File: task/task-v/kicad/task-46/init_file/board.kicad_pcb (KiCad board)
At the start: 2 copper layers, 80 x 80 mm, 8 parts

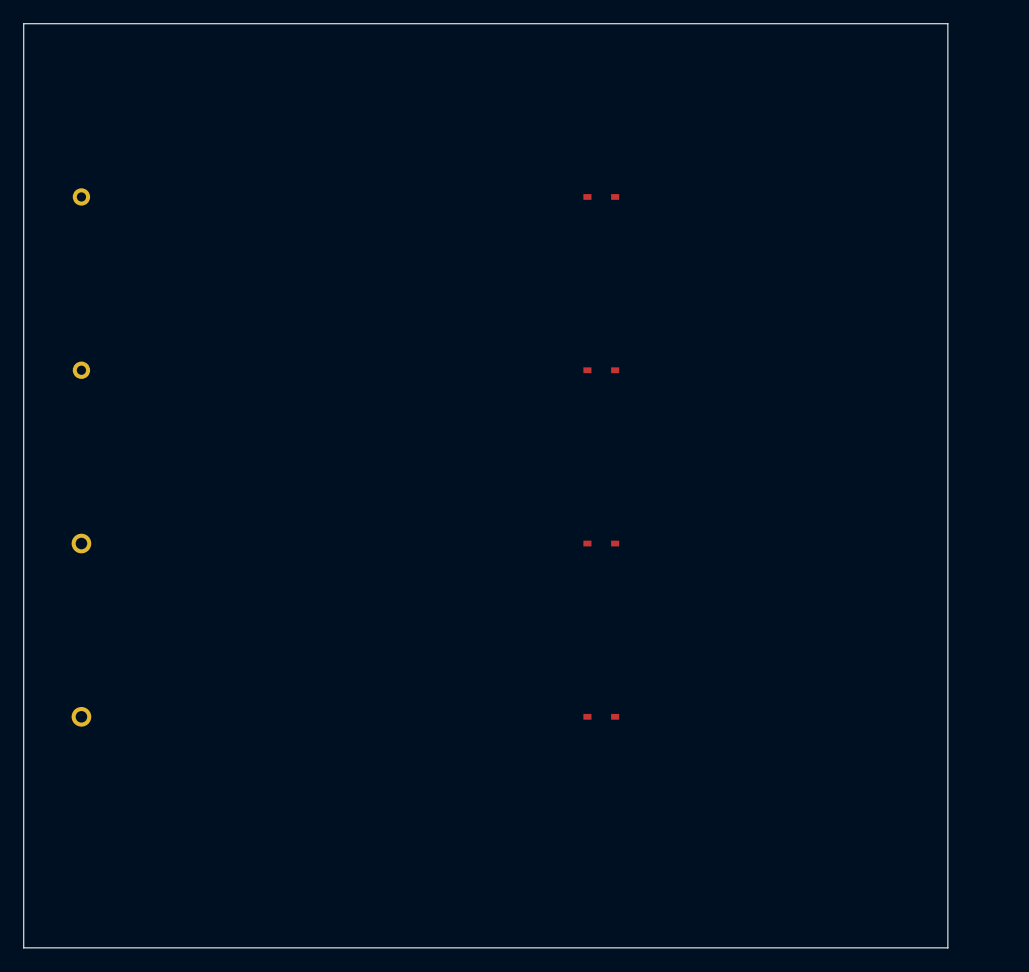
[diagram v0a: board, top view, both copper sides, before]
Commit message: Refine engineering task metadata and instructions
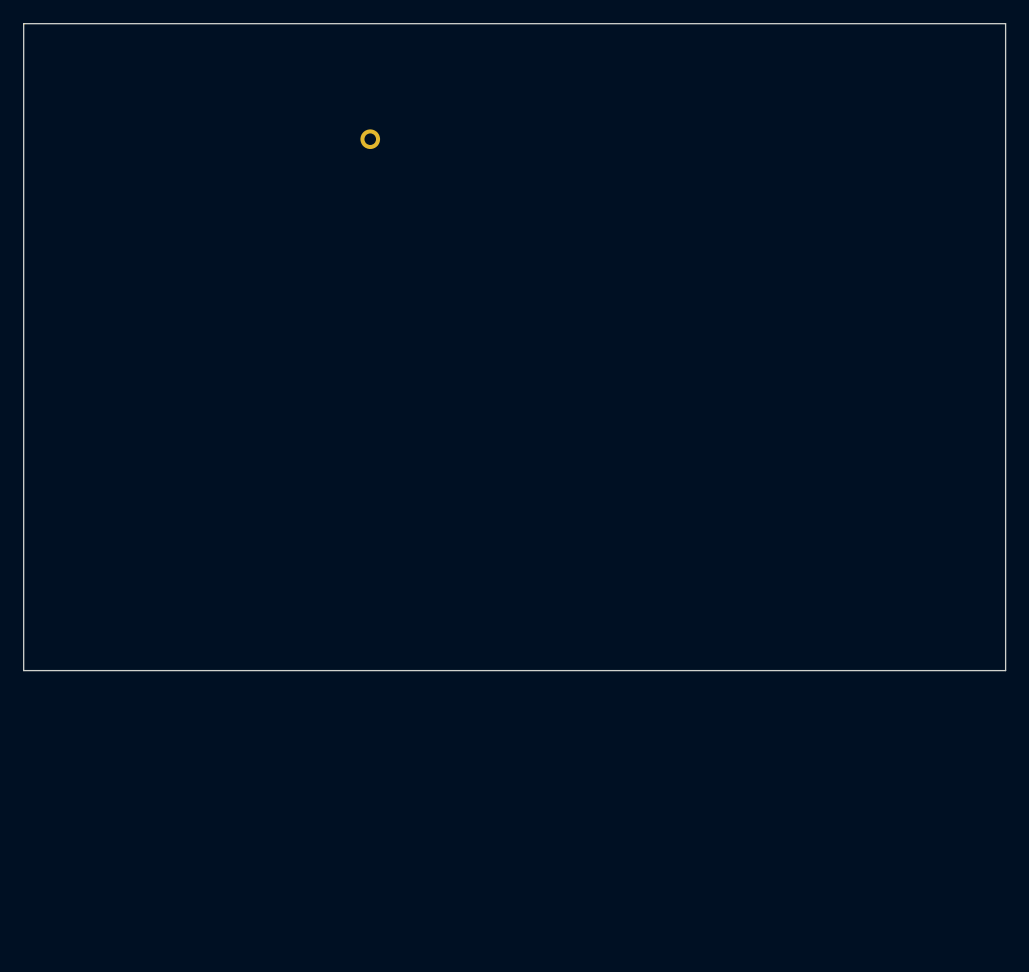
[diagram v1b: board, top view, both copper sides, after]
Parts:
- removed the ? at (5.00, 15.0)
- removed the ? at (5.00, 30.0)
- removed the ? at (5.00, 45.0)
- removed the ? at (5.00, 60.0)
- removed the ? at (50.0, 15.0)
- removed the ? at (50.0, 30.0)
- removed the ? at (50.0, 45.0)
- removed the ? at (50.0, 60.0)
- added ?: , Connector_PinHeader_2.54mm:PinHeader_2x20_P2.54mm_Vertical, F.Cu at (30.0, 10.0)
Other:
- board size 80 x 80 mm -> 85 x 56 mm
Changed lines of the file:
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@@
   )
   (net 0 "")
-  (net 1 "USB_DP")
-  (net 2 "USB_DM")
-  (net 3 "SIG_TX")
-  (net 4 "SIG_RX")
-  (net 5 "GND")
-  ; Connectors at board edge (x=5)
-  (footprint "Connector_USB:USB_A_Molex_67643_Vertical" (layer "F.Cu") (at 5 15)
-    (reference "J1") (value "USB-A")
-    (pad "1" thru_hole circle (at 0 0) (size 1.5 1.5) (drill 0.8)
-      (layers "F.Cu" "B.Cu" "F.Mask" "B.Mask") (net 1 "USB_DP"))
+  (net 1 "VCC")
+  (net 2 "GND")
+  ; Initial board: 85x56mm rectangle, no mounting holes, no rounded corners
+  (gr_rect (start 0 0) (end 85 56) (layer "Edge.Cuts") (width 0.1))
+  ; 2x20 GPIO header at (30, 10) -- needs to be repositioned
+  (footprint "Connector_PinHeader_2.54mm:PinHeader_2x20_P2.54mm_Vertical" (layer "F.Cu") (at 30 10)
+    (reference "J1") (value "GPIO_HEADER")
+    (pad "1" thru_hole circle (at 0 0) (size 1.7 1.7) (drill 1.0)
+      (layers "F.Cu" "B.Cu" "F.Mask" "B.Mask") (net 1 "VCC"))
   )
-  (footprint "Connector_USB:USB_A_Molex_67643_Vertical" (layer "F.Cu") (at 5 30)
-    (reference "J2") (value "USB-A")
-    (pad "1" thru_hole circle (at 0 0) (size 1.5 1.5) (drill 0.8)
-      (layers "F.Cu" "B.Cu" "F.Mask" "B.Mask") (net 2 "USB_DM"))
-  )
-  (footprint "Connector_PinHeader_2.54mm:PinHeader_1x04_P2.54mm_Vertical" (layer "F.Cu") (at 5 45)
-    (reference "J3") (value "CONN-4P")
-    (pad "1" thru_hole circle (at 0 0) (size 1.7 1.7) (drill 1.0)
-      (layers "F.Cu" "B.Cu" "F.Mask" "B.Mask") (net 3 "SIG_TX"))
-  )
-  (footprint "Connector_PinHeader_2.54mm:PinHeader_1x04_P2.54mm_Vertical" (layer "F.Cu") (at 5 60)
-    (reference "J4") (value "CONN-4P")
-    (pad "1" thru_hole circle (at 0 0) (size 1.7 1.7) (drill 1.0)
-      (layers "F.Cu" "B.Cu" "F.Mask" "B.Mask") (net 4 "SIG_RX"))
-  )
-  ; ESD arrays far from connectors (30mm away) — need to be moved
-  (footprint "Package_TO_SOT_SMD:SOT-363_SC-70-6" (layer "F.Cu") (at 50 15)
-    (reference "D1") (value "PRTR5V0U2X")
-    (pad "1" smd rect (at -1.2 0) (size 0.7 0.5)
-      (layers "F.Cu" "F.Paste" "F.Mask") (net 1 "USB_DP"))
-    (pad "6" smd rect (at 1.2 0) (size 0.7 0.5)
-      (layers "F.Cu" "F.Paste" "F.Mask") (net 5 "GND"))
-  )
-  (footprint "Package_TO_SOT_SMD:SOT-363_SC-70-6" (layer "F.Cu") (at 50 30)
-    (reference "D2") (value "PRTR5V0U2X")
-    (pad "1" smd rect (at -1.2 0) (size 0.7 0.5)
-      (layers "F.Cu" "F.Paste" "F.Mask") (net 2 "USB_DM"))
-    (pad "6" smd rect (at 1.2 0) (size 0.7 0.5)
-      (layers "F.Cu" "F.Paste" "F.Mask") (net 5 "GND"))
-  )
-  (footprint "Package_TO_SOT_SMD:SOT-363_SC-70-6" (layer "F.Cu") (at 50 45)
-    (reference "D3") (value "PRTR5V0U2X")
-    (pad "1" smd rect (at -1.2 0) (size 0.7 0.5)
-      (layers "F.Cu" "F.Paste" "F.Mask") (net 3 "SIG_TX"))
-    (pad "6" smd rect (at 1.2 0) (size 0.7 0.5)
-      (layers "F.Cu" "F.Paste" "F.Mask") (net 5 "GND"))
-  )
-  (footprint "Package_TO_SOT_SMD:SOT-363_SC-70-6" (layer "F.Cu") (at 50 60)
-    (reference "D4") (value "PRTR5V0U2X")
-    (pad "1" smd rect (at -1.2 0) (size 0.7 0.5)
-      (layers "F.Cu" "F.Paste" "F.Mask") (net 4 "SIG_RX"))
-    (pad "6" smd rect (at 1.2 0) (size 0.7 0.5)
-      (layers "F.Cu" "F.Paste" "F.Mask") (net 5 "GND"))
-  )
-  (gr_rect (start 0 0) (end 80 80) (layer "Edge.Cuts") (width 0.1))
 )
